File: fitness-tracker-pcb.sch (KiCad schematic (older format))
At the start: 56 parts, among them IC1 BMD-300-A-R, IC2 BQ24230, IC3 TPS63030, IC4 LC709203F, IC5 MMBT2222ALT1G, IC6 DRV2603RUNR, IC7 W25Q128JVPIQ, J1 FH33-4S-1SH_10_, Q1 BC847, U2 BAT-HLD-001, U3 APDS9960, U4 ST7735, U5 nRF52832-QFxx

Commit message: before remove unnecessary parts
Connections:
- net +2V8: now also C21.1
- net BUZZER: now also IC1.31 (P0.13)
- net DISPLAY_BRIGHTNESS: now also IC1.40 (P0.22)
- net DISPLAY_CS: now also IC1.36 (P0.18)
- net DISPLAY_DC: now also IC1.26 (P0.10)
- net DISPLAY_MOSI: now also IC1.28 (P0.12)
- net DISPLAY_RESET: now also IC1.38 (P0.20)
- net DISPLAY_SCK: now also IC1.34 (P0.16)
- net GESTURE_INT: now also IC1.24 (P0.08)
- net GESTURE_SCL: now also IC1.22 (P0.06)
- net GESTURE_SDA: now also IC1.23 (P0.07)
- net GND: now also C21.2
- net IMU_CS: now also IC1.10 (P0.29)
- net IMU_INT1: now also IC1.6 (P0.25)
- net IMU_INT2: now also IC1.11 (P0.30)
- net IMU_MISO: now also IC1.7 (P0.26)
- net IMU_MOSI: now also IC1.8 (P0.27)
- net IMU_SCK: now also IC1.9 (P0.28)
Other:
- moved on the sheet: ANT1, C1, C15, C16, C2, C21, C3, C4, C5, C6, C7, C8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

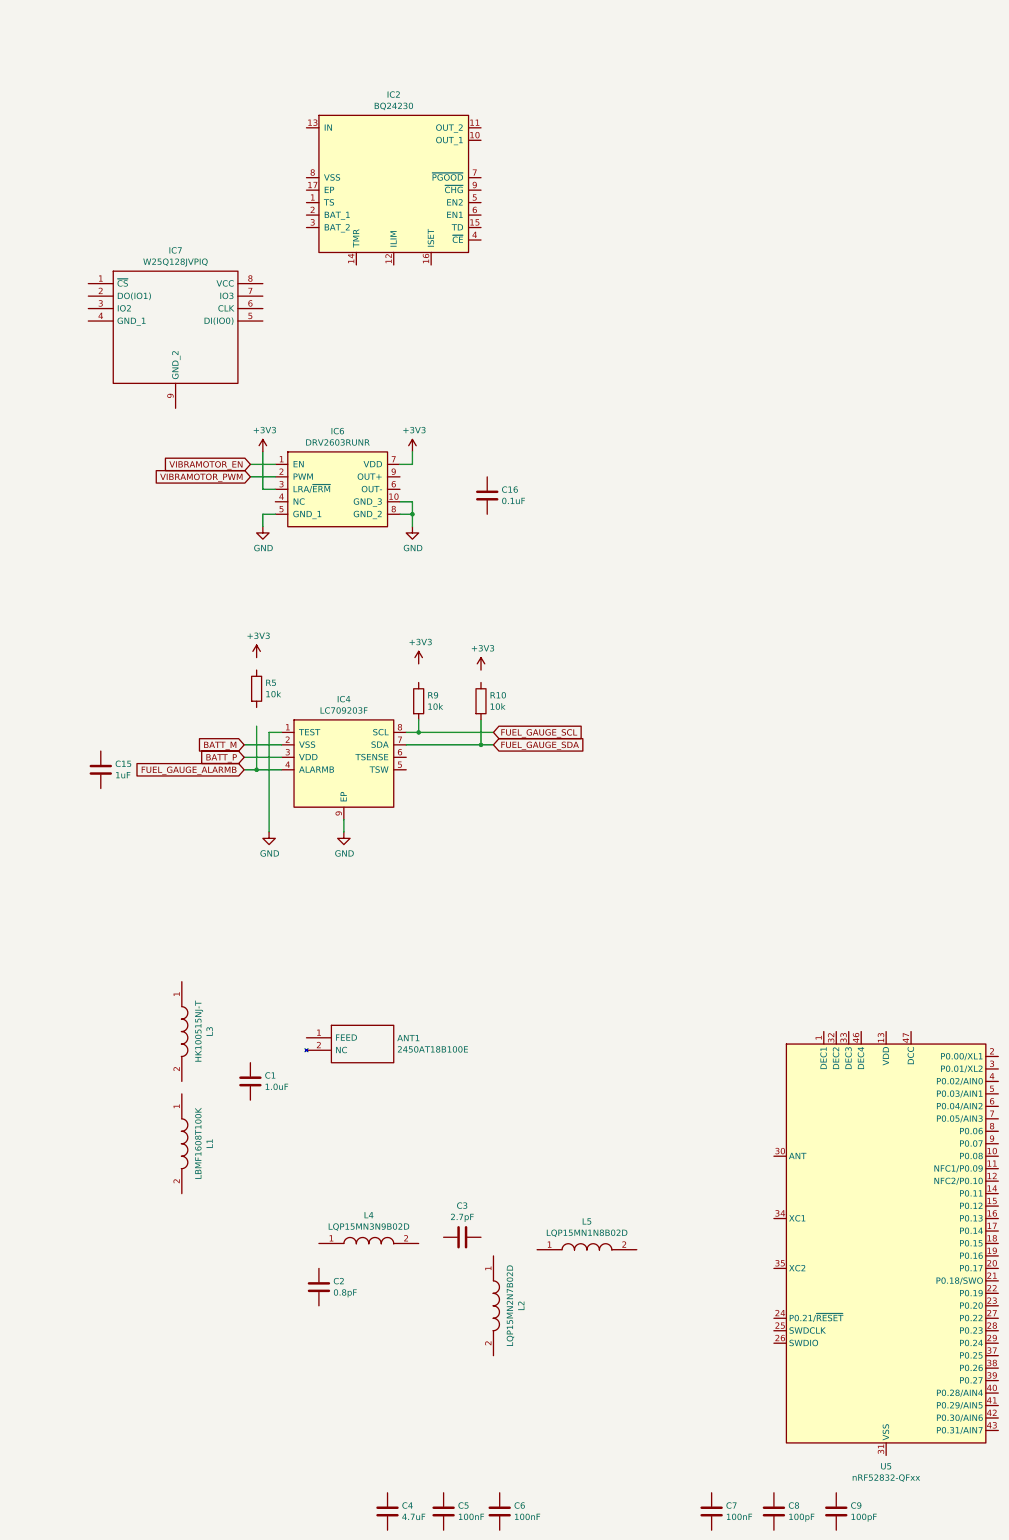
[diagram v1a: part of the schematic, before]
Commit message: almost done 4 layer pcb
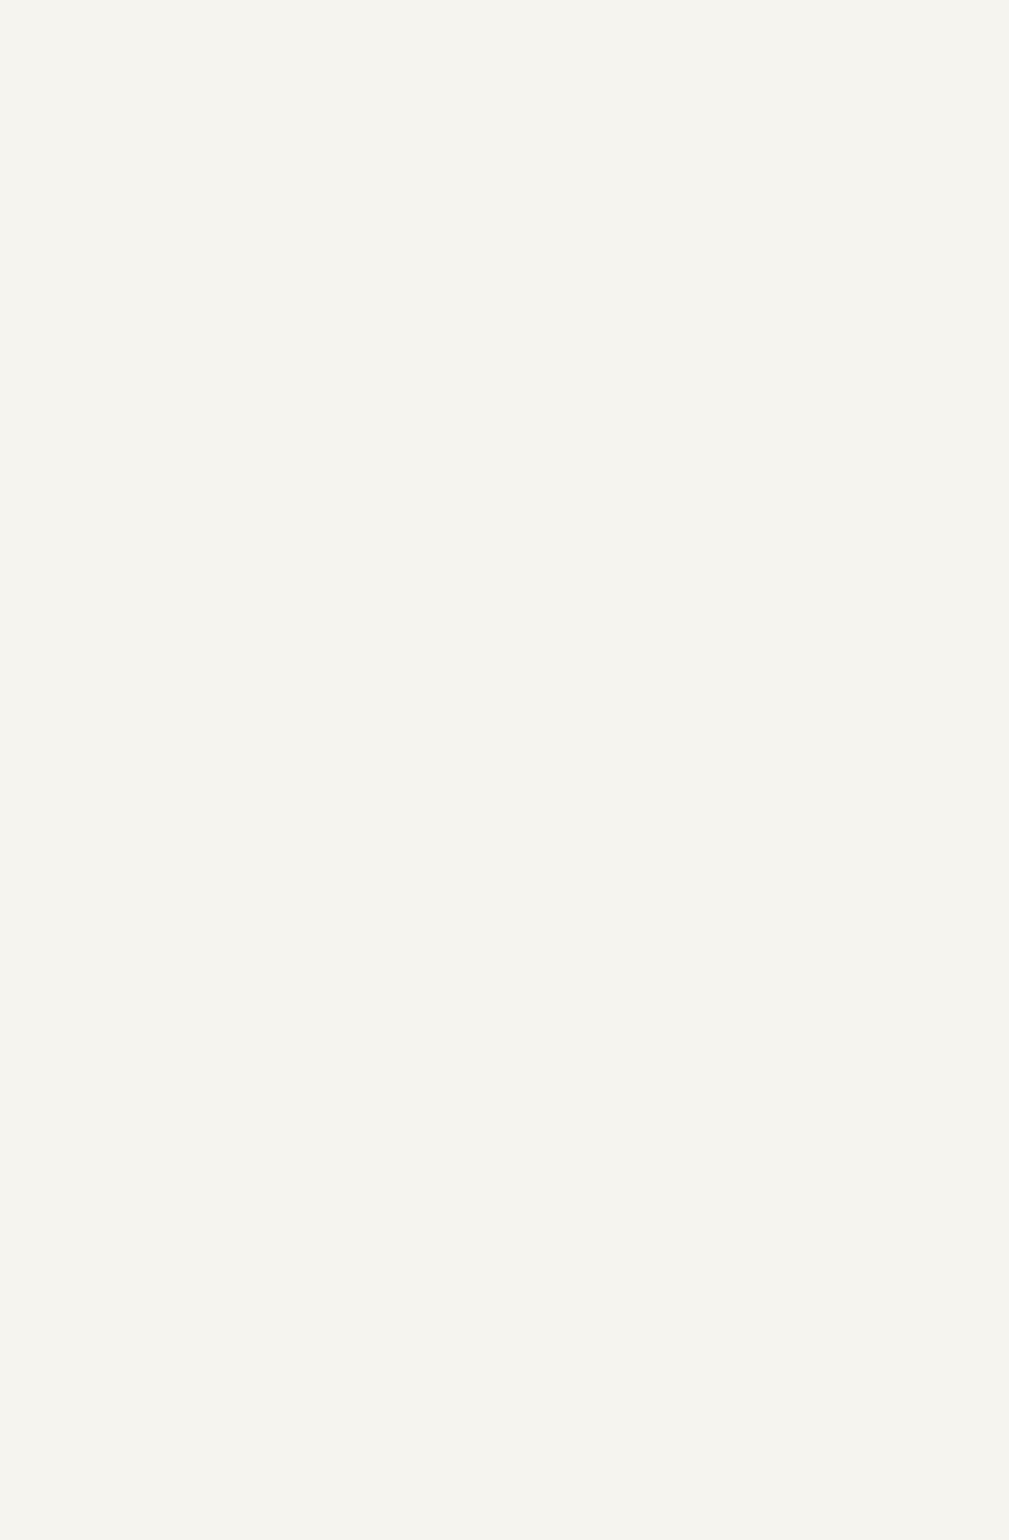
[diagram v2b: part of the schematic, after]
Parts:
- removed ANT1: 2450AT18B100E, ANTC3216X140N, symbol 2450AT18B100E:2450AT18B100E
- removed C1: 1.0uF, Capacitor_SMD:C_0603_1608Metric, symbol Device:C
- removed C15: 1uF, symbol Device:C
- removed C16: 0.1uF, symbol Device:C
- removed C2: 0.8pF, Capacitor_SMD:C_0402_1005Metric, symbol Device:C
- removed C3: 2.7pF, Capacitor_SMD:C_0402_1005Metric, symbol Device:C
- removed C4: 4.7uF, Capacitor_SMD:C_0603_1608Metric, symbol Device:C
- removed C5, C6, C7: 100nF, Capacitor_SMD:C_0402_1005Metric, symbol Device:C
- removed C8, C9: 100pF, Capacitor_SMD:C_0402_1005Metric, symbol Device:C
- removed IC2: BQ24230, BQ24230RGTR:QFN50P300X300X100-17N-D, symbol BQ24230RGTR:BQ24230
- removed IC4: LC709203F, LC709203FQH-01TWG:SON65P400X300X80-9N, symbol LC709203F:LC709203F
- removed IC6: DRV2603RUNR, DRV2603RUNR:QFN50P200X200X80-10N-D, symbol DRV2603RUNR:DRV2603RUNR
- removed IC7: W25Q128JVPIQ, SON127P800X600X80-9N-D, symbol W25Q128JVPIQ:W25Q128JVPIQ
- removed L1: LBMF1608T100K, INDC1608X100N, symbol LBMF1608T100K:LBMF1608T100K
- removed L2: LQP15MN2N7B02D, LQP15MN10NG02D, symbol LQP15MN2N7B02D:LQP15MN2N7B02D
- removed L3: HK100515NJ-T, INDC1005X55N, symbol HK100515NJ-T:HK100515NJ-T
- removed L4: LQP15MN3N9B02D, LQP15MN10NG02D, symbol LQP15MN3N9B02D:LQP15MN3N9B02D
- removed L5: LQP15MN1N8B02D, LQP15MN10NG02D, symbol LQP15MN1N8B02D:LQP15MN1N8B02D
- removed R10, R5, R9: 10k, symbol Device:R
- removed U5: nRF52832-QFxx, Package_DFN_QFN:QFN-48-1EP_6x6mm_P0.4mm_EP4.6x4.6mm, symbol MCU_Nordic:nRF52832-QFxx
